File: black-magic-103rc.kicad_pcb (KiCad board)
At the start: 2 copper layers, 57.9 x 24.2 mm, 69 parts, among them J1 USB_B_Micro, J2 JTAG_SWD_10, J3 UART, J4 SWD_CONN, J5 BOOT0, J6 PORTC, P1 USB_C_Plug_USB2.0, Q1 DMG1024UV, Q2 DMG1023UV, SW1 SW_SPST, U1 USBLC6-2P6, U2 SN74LVC2T45DCUR, U3 STM32F103RCTx, U4 AMS1117-3.3, U5 SN74LVC2T45DCUR, U6 SN74LVC2T45DCUR, U7 SN74LVC2T45DCUR, Y2 8Mhz

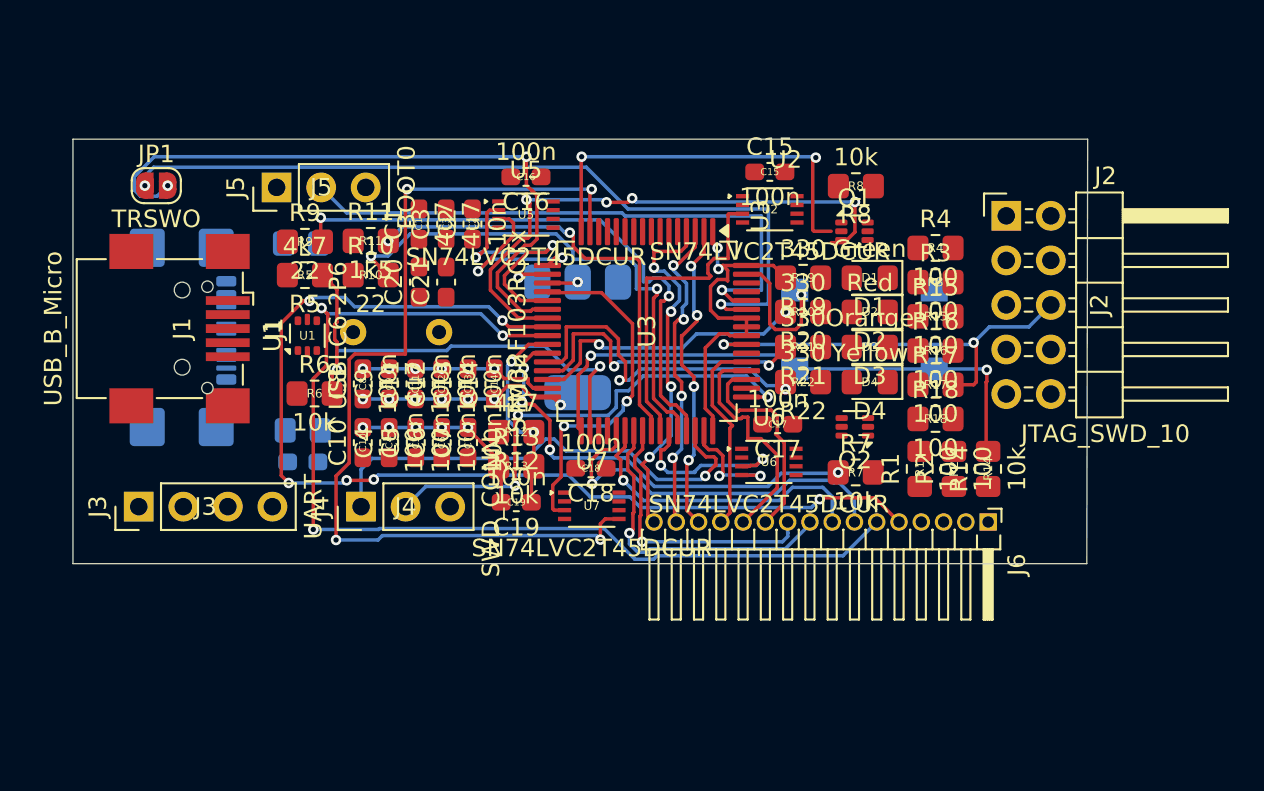
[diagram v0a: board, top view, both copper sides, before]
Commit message: [06-05-1334] update after stagnate
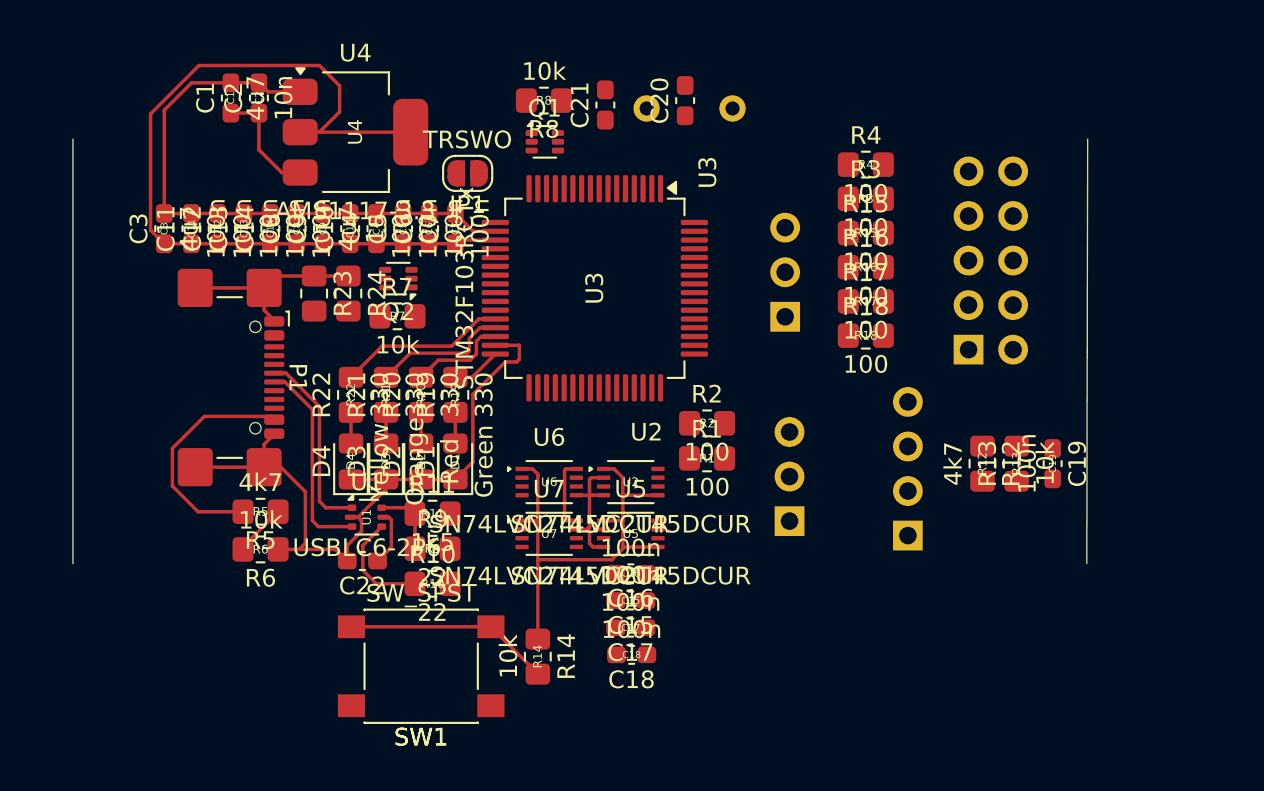
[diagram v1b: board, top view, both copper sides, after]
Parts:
- removed J1: USB_B_Micro, Connector_USB:USB_Mini-B_Wuerth_65100516121_Horizontal
- removed J6: PORTC, Connector_PinHeader_1.27mm:PinHeader_1x16_P1.27mm_Horizontal
- C22, P1, R23, R24, SW1, U4: moved to F.Cu
- J2, J3, J4, J5: moved to B.Cu
- moved J3 43.9 mm to (161.8, 100.5), turned to 0 degrees
- moved SW1 31.7 mm to (134.0, 108.0)
- moved C19 30.7 mm to (170.0, 96.5), turned to -90 degrees
- moved D4 29.9 mm to (130.0, 96.3), turned to 90 degrees
- moved J5 29.9 mm to (154.8, 88.1), turned to 0 degrees
- moved R13 28.5 mm to (168.0, 96.5), turned to 90 degrees
- moved D3 28.3 mm to (132.0, 96.3), turned to 90 degrees
- moved R14 27.8 mm to (140.7, 107.5), turned to -90 degrees
- moved R7 27.6 mm to (132.7, 88.0)
- moved Q2 27.4 mm to (132.7, 85.9)
- moved D2 27.0 mm to (134.0, 96.3), turned to 90 degrees
- moved R12 26.6 mm to (166.0, 96.5), turned to -90 degrees
- moved D1 25.8 mm to (136.0, 96.3), turned to 90 degrees
- moved R22 25.8 mm to (130.0, 92.5), turned to 90 degrees
- moved C15 25.7 mm to (146.0, 104.2), turned to 180 degrees
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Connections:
- U3 pad 10: Net-(J6-Pin_3) -> unconnected-(U3-PC2-Pad10)
- U3 pad 11: Net-(J6-Pin_4) -> unconnected-(U3-PC3-Pad11)
- U3 pad 2: Net-(J6-Pin_14) -> unconnected-(U3-PC13-Pad2)
- U3 pad 24: Net-(J6-Pin_5) -> unconnected-(U3-PC4-Pad24)
- U3 pad 25: Net-(J6-Pin_6) -> unconnected-(U3-PC5-Pad25)
- U3 pad 3: Net-(J6-Pin_15) -> unconnected-(U3-PC14-Pad3)
- U3 pad 37: Net-(J6-Pin_7) -> unconnected-(U3-PC6-Pad37)
- U3 pad 38: Net-(J6-Pin_8) -> unconnected-(U3-PC7-Pad38)
- U3 pad 39: Net-(J6-Pin_9) -> unconnected-(U3-PC8-Pad39)
- U3 pad 4: Net-(J6-Pin_16) -> unconnected-(U3-PC15-Pad4)
- U3 pad 40: Net-(J6-Pin_10) -> unconnected-(U3-PC9-Pad40)
- U3 pad 51: Net-(J6-Pin_11) -> unconnected-(U3-PC10-Pad51)
- U3 pad 52: Net-(J6-Pin_12) -> unconnected-(U3-PC11-Pad52)
- U3 pad 53: Net-(J6-Pin_13) -> unconnected-(U3-PC12-Pad53)
- U3 pad 8: Net-(J6-Pin_1) -> unconnected-(U3-PC0-Pad8)
- U3 pad 9: Net-(J6-Pin_2) -> unconnected-(U3-PC1-Pad9)
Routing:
- net Net-(J6-Pin_5): track 62.3 -> 0.00 mm, vias 6 -> 0
- net Net-(J6-Pin_6): track 60.4 -> 0.00 mm, vias 3 -> 0
- net ITMS_DIR: track 53.7 -> 0.00 mm, vias 4 -> 0
- net GND: track 40.0 -> 92.4 mm, vias 15 -> 0
- net /TRSWO: track 47.0 -> 0.00 mm, vias 2 -> 0
- net +3.3V: track 35.9 -> 78.3 mm, vias 10 -> 0
- net ITDO: track 38.2 -> 0.00 mm, vias 2 -> 0
- net /BOOT0: track 33.9 -> 0.00 mm, vias 1 -> 0
- net /USB+: track 33.0 -> 0.00 mm, vias 2 -> 0
- net IRST_SENSE: track 32.6 -> 0.00 mm, vias 4 -> 0
- net /USB-: track 29.6 -> 0.00 mm, vias 2 -> 0
- net /SWCLK: track 28.2 -> 0.00 mm, vias 3 -> 0
- net /SWDIO: track 27.1 -> 0.00 mm, vias 1 -> 0
- net Net-(U3-PA8): track 25.8 -> 0.00 mm, vias 2 -> 0
- net PWR_BRKOUT: track 25.4 -> 0.00 mm, vias 4 -> 0
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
